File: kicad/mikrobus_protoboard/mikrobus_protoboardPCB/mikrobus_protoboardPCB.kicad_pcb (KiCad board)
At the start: 2 copper layers, 25.2 x 57.2 mm, 0 parts

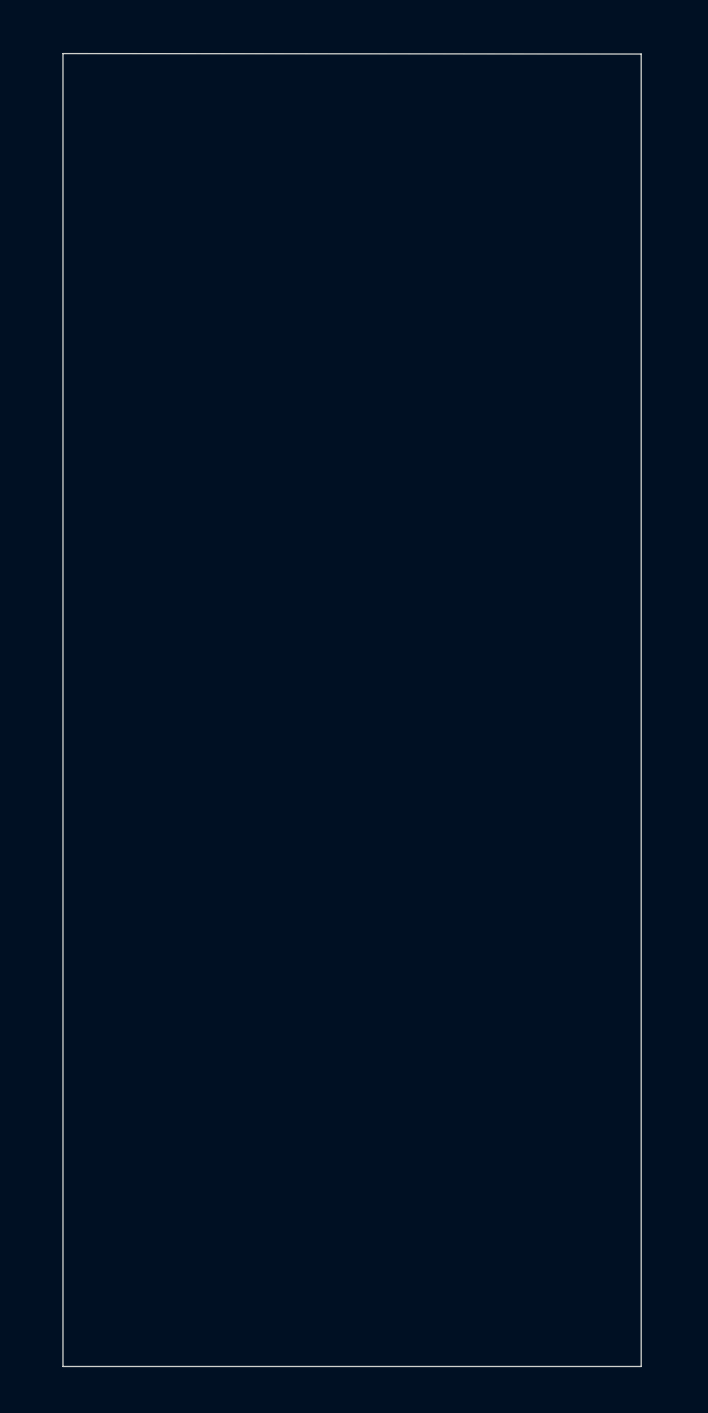
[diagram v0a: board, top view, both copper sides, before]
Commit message: nets complete
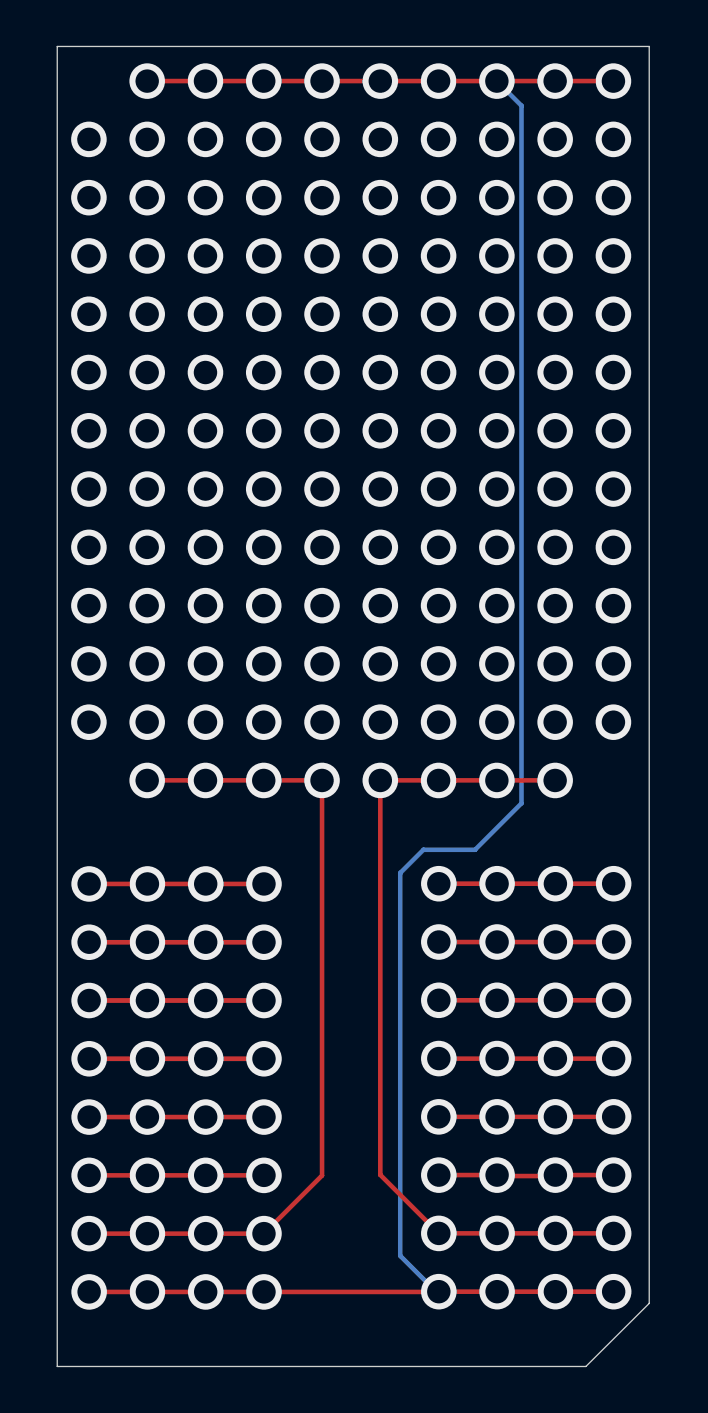
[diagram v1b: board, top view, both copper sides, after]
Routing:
- net GND: track 0.00 -> 100.9 mm, vias 0 -> 17
- net 5V: track 0.00 -> 36.1 mm, vias 0 -> 8
- net 3V3: track 0.00 -> 36.0 mm, vias 0 -> 8
- net SDA: track 0.00 -> 7.69 mm, vias 0 -> 4
- net TX: track 0.00 -> 7.62 mm, vias 0 -> 4
- net SCL: track 0.00 -> 7.62 mm, vias 0 -> 4
- net SCK: track 0.00 -> 7.62 mm, vias 0 -> 4
- net RX: track 0.00 -> 7.62 mm, vias 0 -> 4
- net RST: track 0.00 -> 7.62 mm, vias 0 -> 4
- net PWD: track 0.00 -> 7.62 mm, vias 0 -> 4
- net MOSI: track 0.00 -> 7.62 mm, vias 0 -> 4
- net MISO: track 0.00 -> 7.62 mm, vias 0 -> 4
- net INT: track 0.00 -> 7.62 mm, vias 0 -> 4
- net CS: track 0.00 -> 7.62 mm, vias 0 -> 4
- net AN: track 0.00 -> 7.62 mm, vias 0 -> 4
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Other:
- board size 25.2 x 57.2 mm -> 25.8 x 57.5 mm

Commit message: protoboard ready
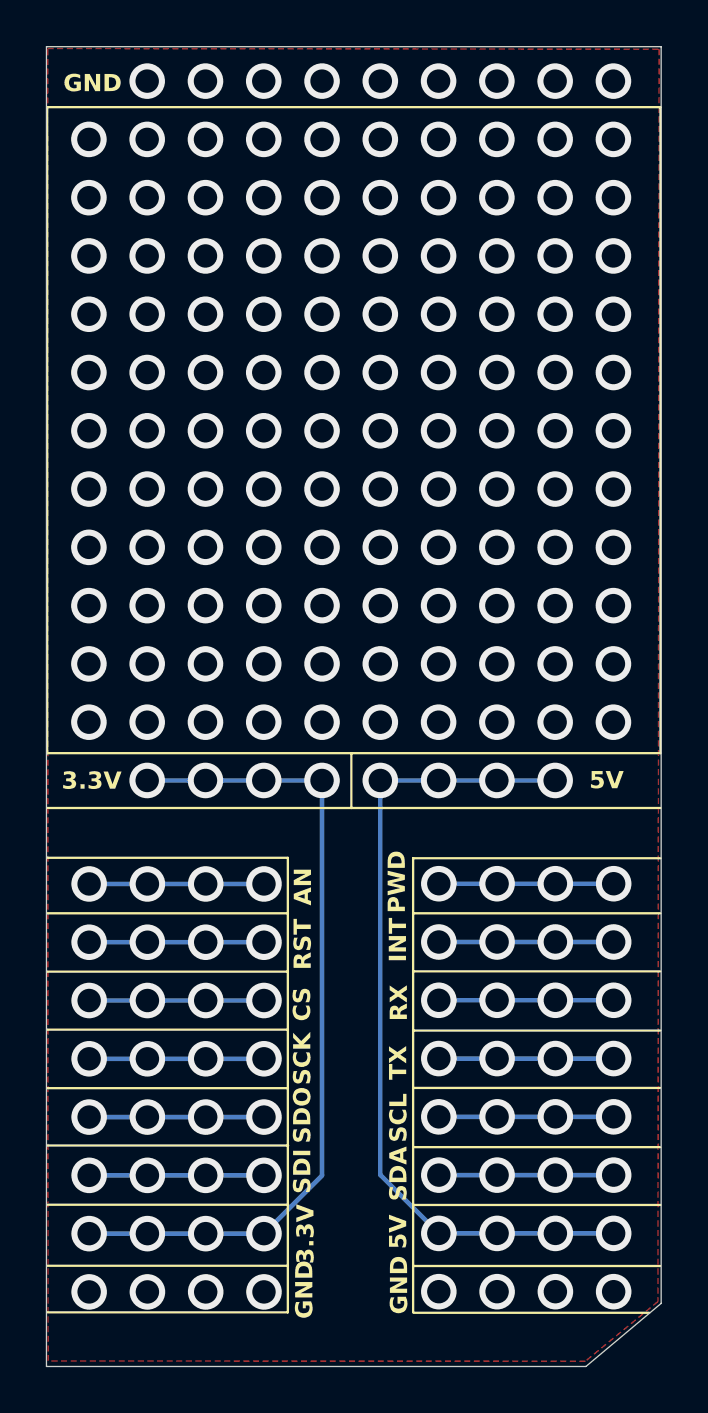
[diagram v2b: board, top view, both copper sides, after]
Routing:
- net GND: track 100.9 -> 0.37 mm
- added copper zone on F.Cu, net GND
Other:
- board size 25.8 x 57.5 mm -> 26.8 x 57.5 mm
- board text added: "3.3V"
- board text added: "5V"
- board text added: "AN"
- board text added: "CS"
- board text added: "GND"
- board text added: "INT"
- board text added: "PWD"
- board text added: "RST"
- board text added: "RX"
- board text added: "SCK"
- board text added: "SCL"
- board text added: "SDA"
- board text added: "SDI"
- board text added: "SDO"
- board text added: "TX"
